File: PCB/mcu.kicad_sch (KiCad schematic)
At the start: 39 parts, among them J101 switch, J102 switch, J103 USB4510-03-1-A, J104 CONN_DISPLAY, U101 W25Q128JVSIQ, U102 RP2040, U103 TPS62172DSG, U104 USBLC6-2SC6, Y101 12MHz

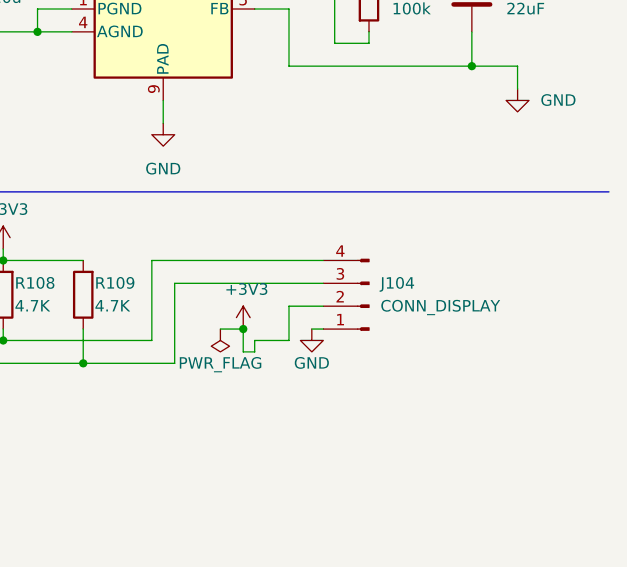
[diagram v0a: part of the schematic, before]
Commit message: add OLED footprint
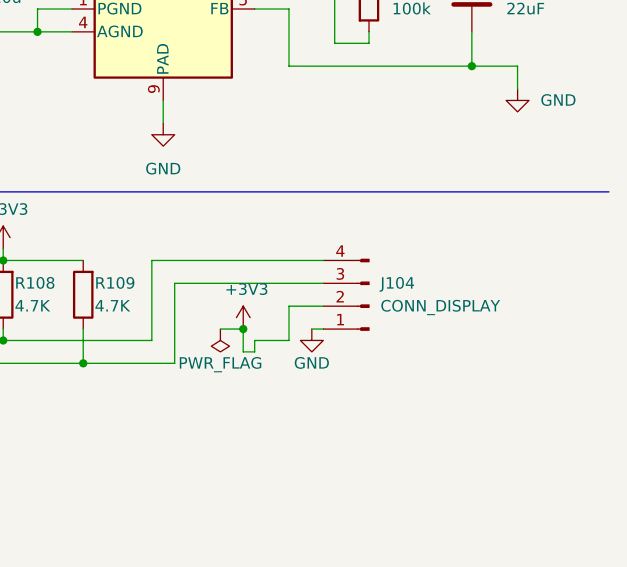
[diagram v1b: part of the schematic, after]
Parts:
- J101: footprint Connector_PinHeader_2.54mm:PinHeader_1x02_P2.54mm_Vertical -> Footprints:SKHLACA010
- J104: footprint Footprints:OLED_128_64 -> Footprints:SSD1306_0.96_Oled
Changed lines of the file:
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@@
     (property "Reference" "J101" (id 0) (at 26.67 22.86 0))
     (property "Value" "switch" (id 1) (at 27.94 29.21 0))
-    (property "Footprint" "Connector_PinHeader_2.54mm:PinHeader_1x02_P2.54mm_Vertical" (id 2) (at 27.94 21.59 0)
+    (property "Footprint" "Footprints:SKHLACA010" (id 2) (at 27.94 21.59 0)
       (effects (font (size 1.27 1.27)) hide)
     )
@@
   )
   (symbol (lib_id "Connector:Conn_01x04_Male") (at 257.81 157.48 180) (unit 1)
-    (in_bom yes) (on_board yes) (fields_autoplaced)
-    (property "Reference" "J104" (id 0) (at 259.08 154.9399 0)
+    (in_bom yes) (on_board yes)
+    (property "Reference" "J104" (id 0) (at 259.08 154.94 0)
       (effects (font (size 1.27 1.27)) (justify right))
     )
@@
       (effects (font (size 1.27 1.27)) (justify right))
     )
-    (property "Footprint" "Footprints:OLED_128_64" (id 2) (at 257.81 157.48 0)
-      (effects (font (size 1.27 1.27)) hide)
-    )
+    (property "Footprint" "Footprints:SSD1306_0.96_Oled" (id 2) (at 257.81 157.48 0)
+      (effects (font (size 1.27 1.27)) hide)
+    )
